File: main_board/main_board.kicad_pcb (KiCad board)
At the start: 2 copper layers, 160 x 110 mm, 152 parts, among them IC1 MP2722GRH-0000-Z, IC2 MP3429GL-Z, IC4 TS921ID, IC5 CY7C65632-28LTXC, IC6 TS921ID, J1 USB3_A, J10 Conn_01x22_Female, J11 501568-0607-TR325, J12 SM04B-XSRS-ETBLFSN, J13 SM10B-XSRS-ETB, J2 USB3_A, J22 690-019-298-412, J3 Bus_M.2_Socket_M, J4 USB_B_Micro, J5 USB_C_Receptacle_USB2.0, J6 USB_A, J7 USB_A, J8 AudioJack3, J9 The_card, U1 AP3441SHE-7B, U12 RT9742SNGV, U2 ASEK-32.768KHZ-L-R-T, U3 ATmega32U4-M, U4 AP22653W6, U5 AP2204RB-3.3, U6 AP22653W6, U7 INA220AIDGST, U8 STUSB4500QTR, Y1 Crystal, Y2 12MHz

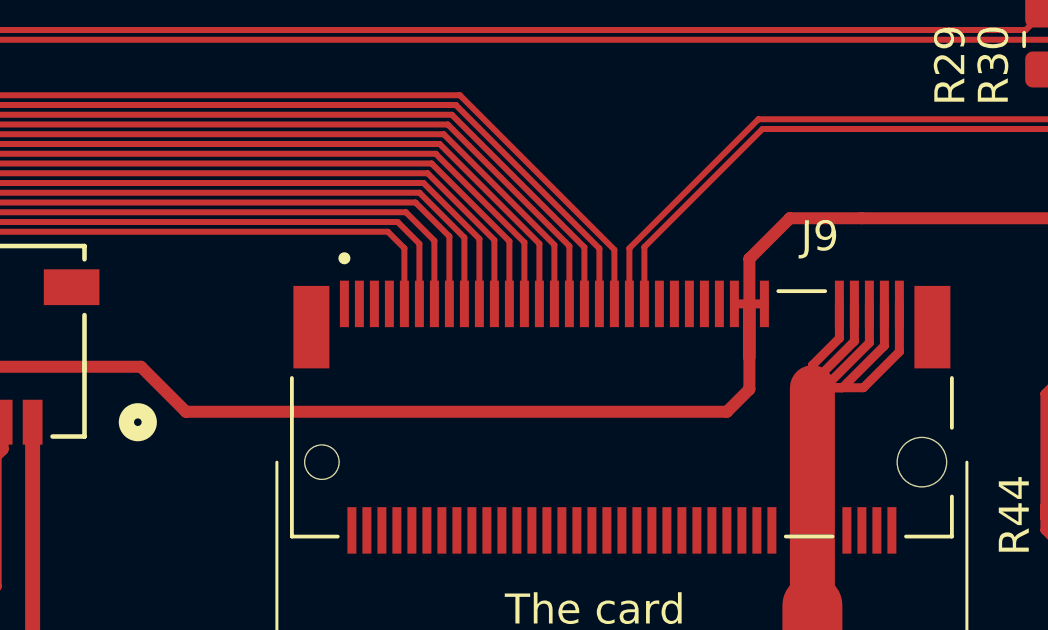
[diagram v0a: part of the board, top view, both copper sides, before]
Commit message: More ground improvements
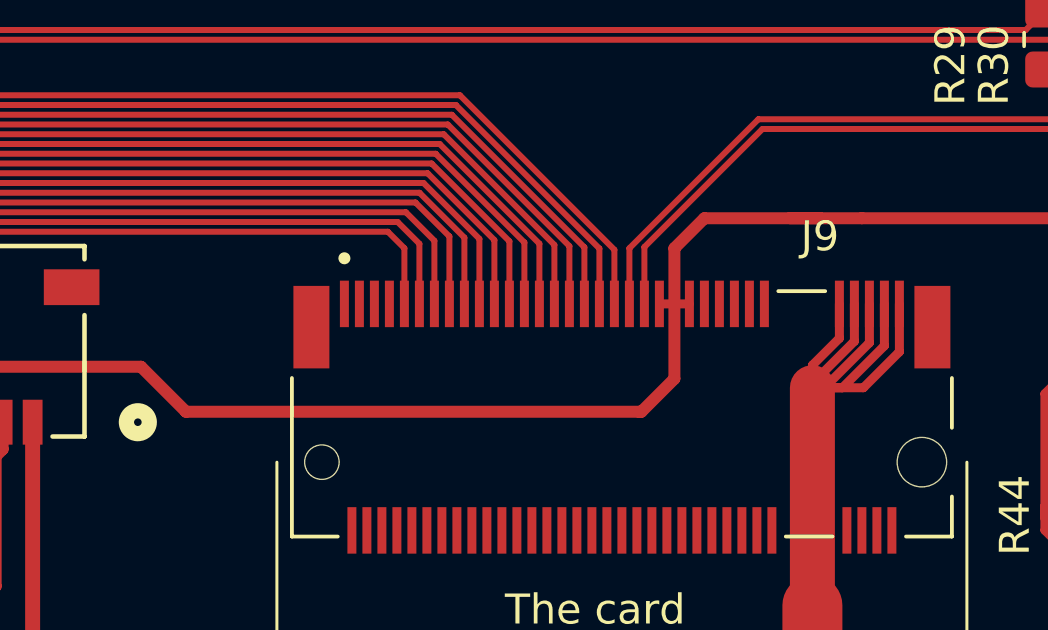
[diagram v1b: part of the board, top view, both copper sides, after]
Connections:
- J9 pad 43: GND -> /CM5_GPIO/+3.3v
- J9 pad 45: GND -> /CM5_GPIO/+3.3v
- J9 pad 47: GND -> /CM5_GPIO/+3.3v
- J9 pad 53: /CM5_GPIO/+3.3v -> GND
- J9 pad 55: /CM5_GPIO/+3.3v -> GND
- J9 pad 57: /CM5_GPIO/+3.3v -> GND
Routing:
- net /CM5_GPIO/+3.3v: track 255.9 -> 255.1 mm
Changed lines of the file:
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@@
 			(size 0.3 1.55)
 			(layers "F.Cu" "F.Paste" "F.Mask")
-			(net 1 "GND")
+			(net 26 "/CM5_GPIO/+3.3v")
 			(pintype "bidirectional")
 			(solder_mask_margin 0.102)
@@
 			(size 0.3 1.55)
 			(layers "F.Cu" "F.Paste" "F.Mask")
-			(net 1 "GND")
+			(net 26 "/CM5_GPIO/+3.3v")
 			(pintype "bidirectional")
 			(solder_mask_margin 0.102)
@@
 			(size 0.3 1.55)
 			(layers "F.Cu" "F.Paste" "F.Mask")
-			(net 1 "GND")
+			(net 26 "/CM5_GPIO/+3.3v")
 			(pintype "bidirectional")
 			(solder_mask_margin 0.102)
@@
 			(size 0.3 1.55)
 			(layers "F.Cu" "F.Paste" "F.Mask")
-			(net 26 "/CM5_GPIO/+3.3v")
+			(net 1 "GND")
 			(pintype "bidirectional")
 			(solder_mask_margin 0.102)
@@
 			(size 0.3 1.55)
 			(layers "F.Cu" "F.Paste" "F.Mask")
-			(net 26 "/CM5_GPIO/+3.3v")
+			(net 1 "GND")
 			(pintype "bidirectional")
 			(solder_mask_margin 0.102)
@@
 			(size 0.3 1.55)
 			(layers "F.Cu" "F.Paste" "F.Mask")
-			(net 26 "/CM5_GPIO/+3.3v")
+			(net 1 "GND")
 			(pintype "bidirectional")
 			(solder_mask_margin 0.102)
@@
 	)
 	(segment
-		(start 143.45 75.255)
-		(end 144.45 75.255)
-		(width 0.3)
-		(layer "F.Cu")
-		(net 26)
-	)
-	(segment
-		(start 143.95 75.255)
-		(end 143.95 78.1)
-		(width 0.4)
-		(layer "F.Cu")
-		(net 26)
-	)
-	(segment
 		(start 155.8 83.3)
 		(end 154.3 83.3)
@@
 	)
 	(segment
-		(start 143.95 75.255)
-		(end 143.95 73.75)
-		(width 0.4)
-		(layer "F.Cu")
-		(net 26)
-	)
-	(segment
 		(start 157.675 80.3625)
 		(end 157.675 79.875)
@@
 	)
 	(segment
-		(start 143.2 78.85)
-		(end 125.17 78.85)
+		(start 141.45 77.75)
+		(end 141.45 75.255)
 		(width 0.4)
 		(layer "F.Cu")
@@
 	)
 	(segment
+		(start 140.95 75.255)
+		(end 141.95 75.255)
+		(width 0.3)
+		(layer "F.Cu")
+		(net 26)
+	)
+	(segment
 		(start 115.125 51.275)
 		(end 115.75 50.65)
@@
 	)
 	(segment
+		(start 145.3 72.4)
+		(end 146.3 72.4)
+		(width 0.4)
+		(layer "F.Cu")
+		(net 26)
+	)
+	(segment
 		(start 157.675 83.3625)
 		(end 157.1375 83.3625)
@@
 	)
 	(segment
+		(start 146.3 72.4)
+		(end 142.45 72.4)
+		(width 0.4)
+		(layer "F.Cu")
+		(net 26)
+	)
+	(segment
 		(start 176.125 90.2)
 		(end 176.75 90.825)
@@
 	)
 	(segment
-		(start 143.95 78.1)
-		(end 143.2 78.85)
+		(start 91.525 85.675)
+		(end 87.25 81.4)
 		(width 0.4)
 		(layer "F.Cu")
@@
 	)
 	(segment
-		(start 91.525 85.675)
-		(end 87.25 81.4)
+		(start 146.3 72.4)
+		(end 147.7 72.4)
 		(width 0.4)
 		(layer "F.Cu")
@@
 	)
 	(segment
-		(start 143.95 73.75)
-		(end 145.3 72.4)
+		(start 140.35 78.85)
+		(end 141.45 77.75)
 		(width 0.4)
 		(layer "F.Cu")
@@
 	)
 	(segment
-		(start 93.4 60.25)
-		(end 93.4 61.141)
-		(width 0.2)
+		(start 140.275 78.85)
+		(end 125.17 78.85)
+		(width 0.4)
 		(layer "F.Cu")
 		(net 26)
 	)
 	(segment
-		(start 143.95 77.05)
-		(end 143.95 75.255)
-		(width 0.4)
+		(start 93.4 60.25)
+		(end 93.4 61.141)
+		(width 0.2)
 		(layer "F.Cu")
 		(net 26)
@@
 	)
 	(segment
+		(start 142.45 72.4)
+		(end 141.45 73.4)
+		(width 0.4)
+		(layer "F.Cu")
+		(net 26)
+	)
+	(segment
 		(start 94.221 59.9)
 		(end 94.221 60.091)
@@
 	)
 	(segment
+		(start 140.275 78.85)
+		(end 140.35 78.85)
+		(width 0.4)
+		(layer "F.Cu")
+		(net 26)
+	)
+	(segment
 		(start 113.8 77.35)
 		(end 105.475 85.675)
@@
 	)
 	(segment
-		(start 145.3 72.4)
-		(end 147.7 72.4)
-		(width 0.4)
+		(start 153.8 82)
+		(end 153.8 82.4)
+		(width 0.3)
 		(layer "F.Cu")
 		(net 26)
 	)
 	(segment
-		(start 153.8 82)
-		(end 153.8 82.4)
-		(width 0.3)
+		(start 141.45 73.4)
+		(end 141.45 75.255)
+		(width 0.4)
 		(layer "F.Cu")
 		(net 26)
